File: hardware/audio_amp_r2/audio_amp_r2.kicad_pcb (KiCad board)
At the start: 2 copper layers, 92 x 35 mm, 32 parts, among them J1 PJ-320D, J2 PJ-320D, J3 JST_PH_1x02, J6 KH-BNC50-3511, J7 KH-BNC50-3511, J8 Conn_01x04_Pin, U1 AD8397, U2 AMS1117-3.3

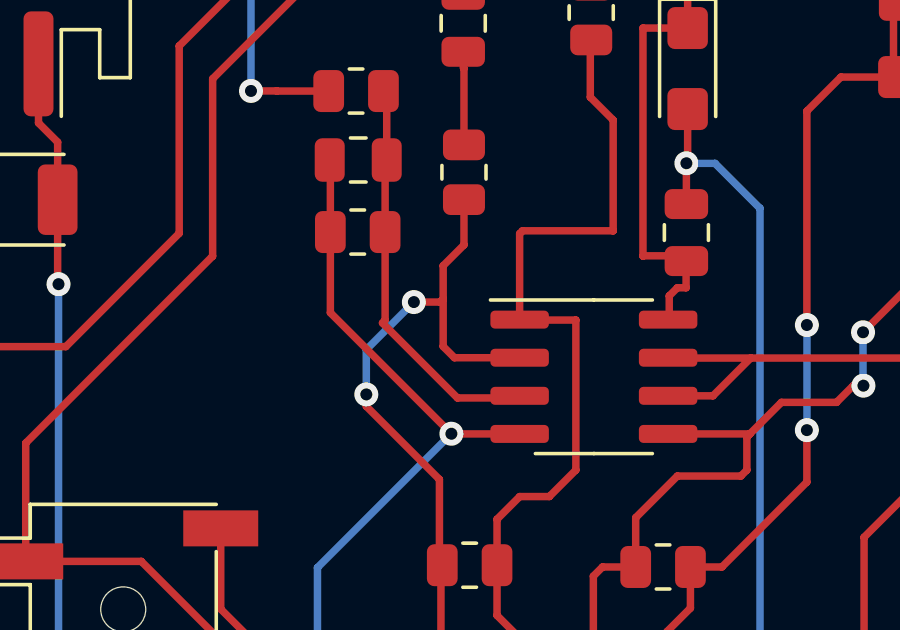
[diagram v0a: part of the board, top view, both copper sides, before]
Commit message: version sent for R2build of audio amp HW
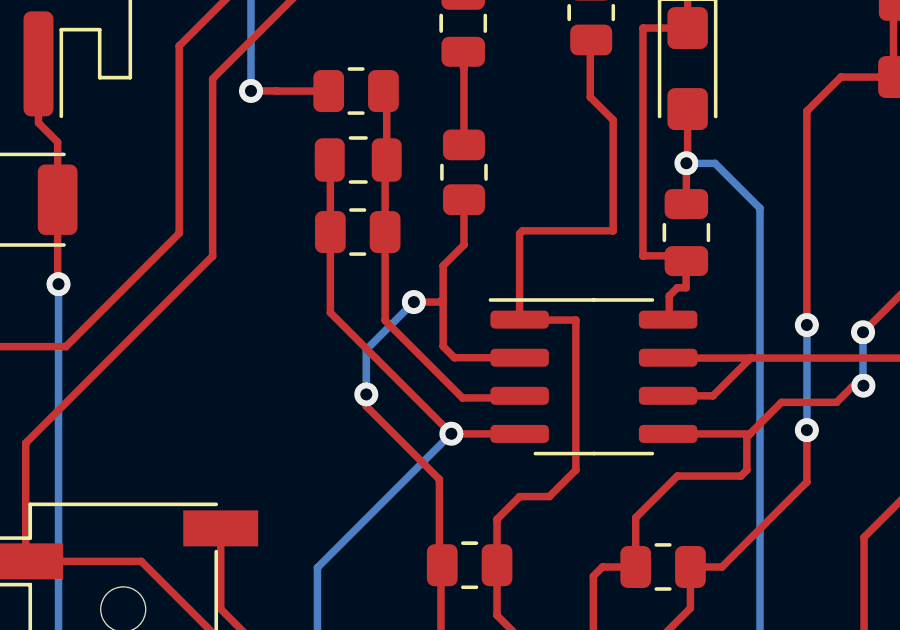
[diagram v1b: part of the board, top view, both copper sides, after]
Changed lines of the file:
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@@
     (descr "SOIC, 8 Pin (JEDEC MS-012AA, https://www.analog.com/media/en/package-pcb-resources/package/pkg_pdf/soic_narrow-r/r_8.pdf), generated with kicad-footprint-generator ipc_gullwing_generator.py")
     (tags "SOIC SO")
-    (property "JLCPCB Part #" "C578714")
+    (property "JLCPCB Part #" "C90876")
     (property "Sheetfile" "audio_amp_r2.kicad_sch")
     (property "Sheetname" "")
@@
     (property "Sim.Enable" "0")
     (property "dnp" "")
-    (property "exclude_from_bom" "")
     (property "ki_description" "Generic connector, single row, 01x04, script generated")
     (property "ki_keywords" "connector")
-    (attr through_hole exclude_from_bom)
+    (attr through_hole)
     (fp_text reference "J8" (at 0 -2.33 90) (layer "F.SilkS") hide
         (effects (font (size 1 1) (thickness 0.15)))
@@
   (segment (start 79.348243 126.082174) (end 79.348243 123.52968) (width 0.25) (layer "F.Cu") (net 8))
   (segment (start 79.348243 123.52968) (end 79.322678 123.504115) (width 0.25) (layer "F.Cu") (net 8))
+  (segment (start 81.13279 134.51738) (end 81.20345 134.44672) (width 0.25) (layer "F.Cu") (net 9))
+  (segment (start 76.719456 131.937454) (end 79.299382 134.51738) (width 0.25) (layer "F.Cu") (net 9))
   (segment (start 76.773565 124.39757) (end 76.663862 124.287867) (width 0.25) (layer "F.Cu") (net 9))
   (segment (start 76.773565 126.585927) (end 76.773565 124.39757) (width 0.25) (layer "F.Cu") (net 9))
-  (segment (start 81.13279 134.51738) (end 81.20345 134.44672) (width 0.25) (layer "F.Cu") (net 9))
-  (segment (start 79.131352 134.51738) (end 81.13279 134.51738) (width 0.25) (layer "F.Cu") (net 9))
-  (segment (start 76.719456 131.930484) (end 76.631956 132.017984) (width 0.25) (layer "F.Cu") (net 9))
+  (segment (start 76.719456 128.987867) (end 76.719456 131.937454) (width 0.25) (layer "F.Cu") (net 9))
   (segment (start 76.719456 128.987867) (end 76.719456 126.640036) (width 0.25) (layer "F.Cu") (net 9))
-  (segment (start 76.719456 128.987867) (end 76.719456 131.930484) (width 0.25) (layer "F.Cu") (net 9))
-  (segment (start 76.631956 132.017984) (end 79.131352 134.51738) (width 0.25) (layer "F.Cu") (net 9))
+  (segment (start 79.299382 134.51738) (end 81.13279 134.51738) (width 0.25) (layer "F.Cu") (net 9))
   (segment (start 90.778017 137.321191) (end 87.94729 140.151918) (width 0.25) (layer "F.Cu") (net 10))
   (segment (start 86.897221 140.151918) (end 86.897221 141.524238) (width 0.25) (layer "F.Cu") (net 10))
